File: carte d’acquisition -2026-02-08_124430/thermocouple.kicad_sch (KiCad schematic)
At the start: 6 parts, among them U6 MAX31855SASA_T, U7 MC74HC4067ADWR2G, U8 MC74HC4067ADWR2G

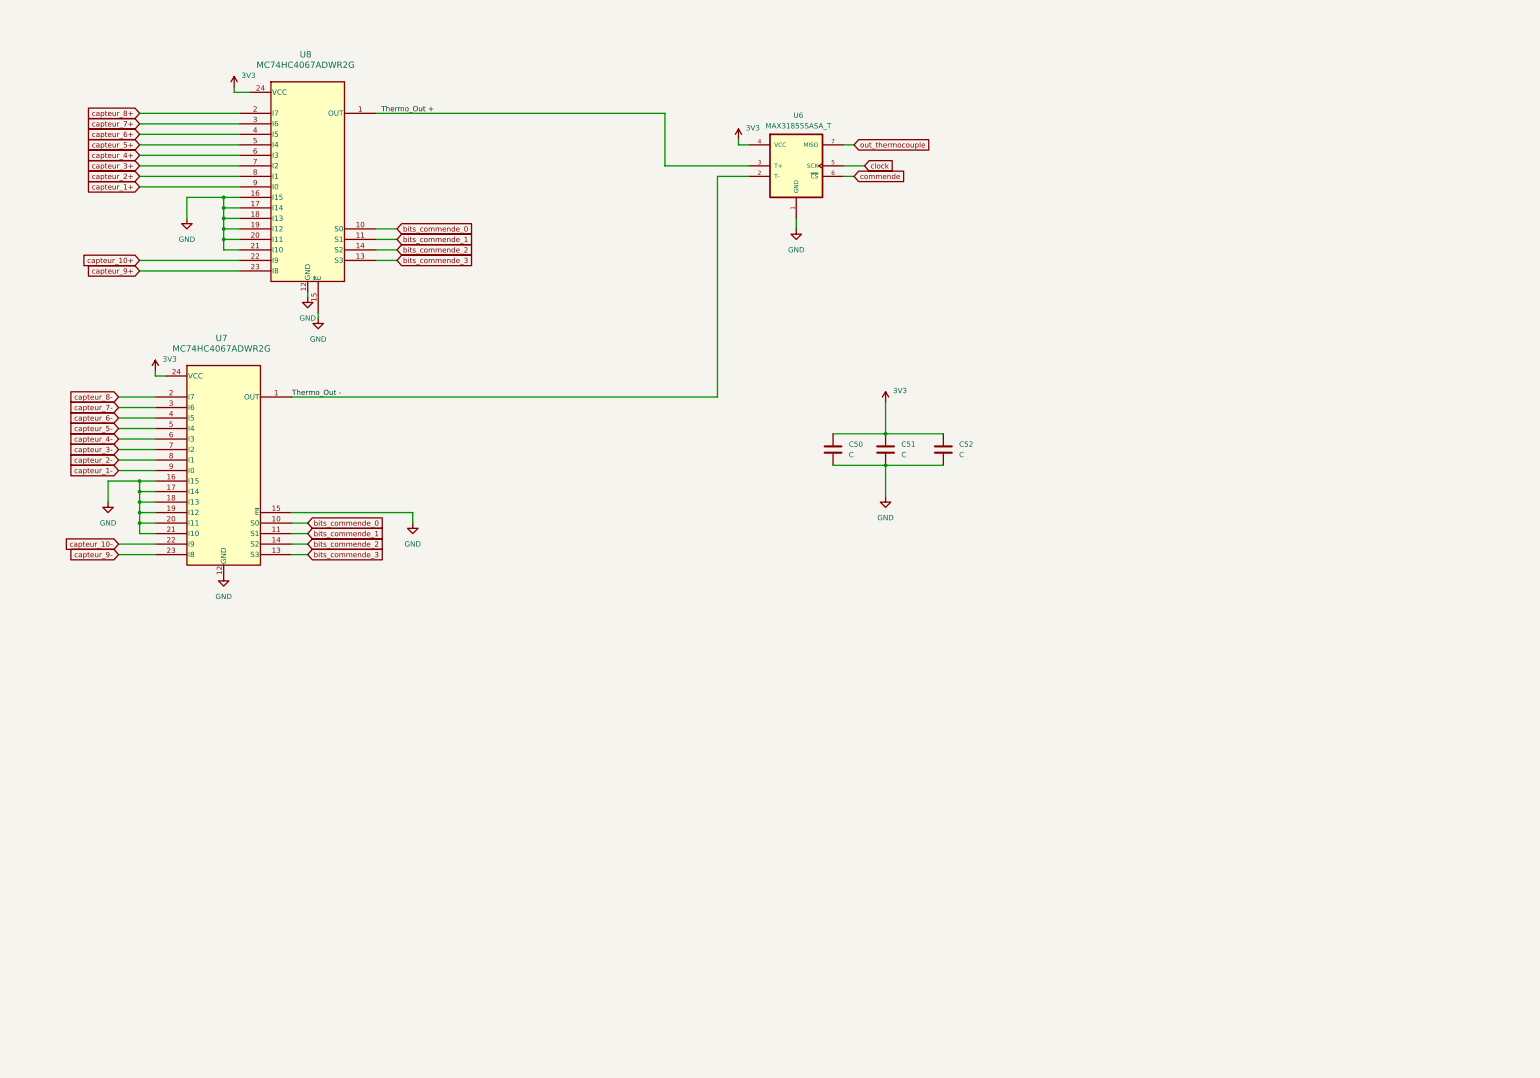
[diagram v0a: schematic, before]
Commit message: arthur net
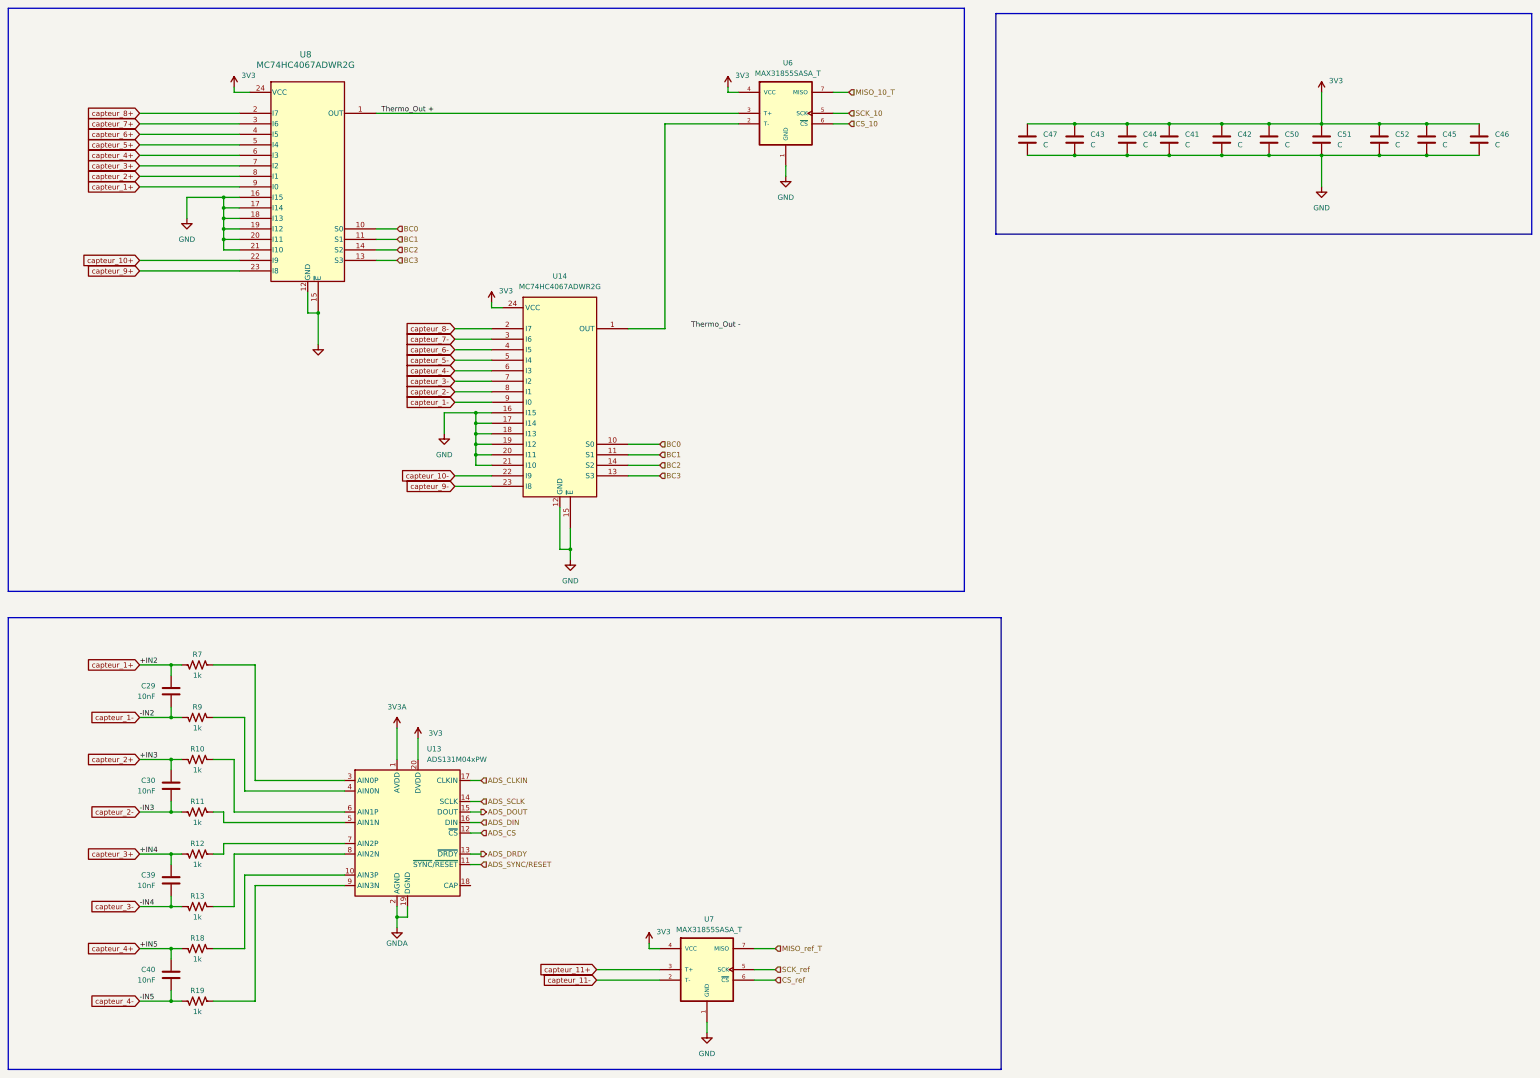
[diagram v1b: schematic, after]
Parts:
- removed U7: MC74HC4067ADWR2G, footprints:SOIC-24WB_ONS, symbol MC74HC4067ADWR2G:MC74HC4067ADWR2G
- added C29, C30, C39, C40: 10nF, symbol Device:C
- added C41, C42, C43, C44, C45, C46, C47: C, symbol Device:C
- added R10, R11, R12, R13, R18, R19, R7, R9: 1k, symbol Device:R_US
- added U13: ADS131M04xPW, Package_SO:TSSOP-20_4.4x6.5mm_P0.65mm, symbol Analog_ADC:ADS131M04xPW
- added U14: MC74HC4067ADWR2G, Package_SO:SOIC-24W_7.5x15.4mm_P1.27mm, symbol FSU_LIB:MC74HC406
- added U7: MAX31855SASA_T, MAX31855SASA_T:SOIC127P600X175-8N, symbol MAX31855SASA_T:MAX31855SASA_T
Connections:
- net 3V3: now also C41.1, C42.1, C43.1, C44.1, C45.1, C46.1, C47.1, U13.20 (DVDD), U14.24 (VCC), U7.4 (VCC)
- net GND: now also C41.2, C42.2, C43.2, C44.2, C45.2, C46.2, C47.2, U14.12 (GND), U14.15 (~{E}), U14.16 (I15), U14.17 (I14), U14.18 (I13), U14.19 (I12), U14.20 (I11), U14.21 (I10), U7.1 (GND)
- net Thermo_Out -: no longer U6.2 (T-)
- net capteur_1+: now also C29.2, R7.2
- net capteur_1-: now also C29.1, R9.2, U14.9 (I0)
- net capteur_10-: now also U14.22 (I9)
- net capteur_2+: now also C30.2, R10.2
- net capteur_2-: now also C30.1, R11.2, U14.8 (I1)
- net capteur_3+: now also C39.2, R12.2
- net capteur_3-: now also C39.1, R13.2, U14.7 (I2)
- net capteur_4+: now also C40.2, R18.2
- net capteur_4-: now also C40.1, R19.2, U14.6 (I3)
- net capteur_5-: now also U14.5 (I4)
- net capteur_6-: now also U14.4 (I5)
- net capteur_7-: now also U14.3 (I6)
- net capteur_8-: now also U14.2 (I7)
- net capteur_9-: now also U14.23 (I8)
- net bits_commende_0 renamed BC0
- net BC0: now also U14.10 (S0)
- net bits_commende_1 renamed BC1
- net BC1: now also U14.11 (S1)
- net bits_commende_2 renamed BC2
- net BC2: now also U14.14 (S2)
- net bits_commende_3 renamed BC3
- net BC3: now also U14.13 (S3)
- net clock renamed SCK_10
- net commende renamed CS_10
- net out_thermocouple renamed MISO_10_T
- new net: R7.1, U13.3 (AIN0P)
- new net: R18.1, U13.10 (AIN3P)
- new net: R9.1, U13.4 (AIN0N)
- new net: R11.1, U13.5 (AIN1N)
- new net: R10.1, U13.6 (AIN1P)
- new net: R12.1, U13.7 (AIN2P)
- new net: R13.1, U13.8 (AIN2N)
- new net: R19.1, U13.9 (AIN3N)
- new net: U14.1 (OUT), U6.2 (T-)
- new net 3V3A: U13.1 (AVDD)
- new net ADS_CLKIN: U13.17 (CLKIN)
- new net ADS_CS: U13.12 (~{CS})
- new net ADS_DIN: U13.16 (DIN)
- new net ADS_DOUT: U13.15 (DOUT)
- new net ADS_DRDY: U13.13 (~{DRDY})
- new net ADS_SCLK: U13.14 (SCLK)
- new net ADS_SYNC/RESET: U13.11 (~{SYNC}/~{RESET})
- new net CS_ref: U7.6 (~{CS})
- new net GNDA: U13.19 (DGND), U13.2 (AGND)
- new net MISO_ref_T: U7.7 (MISO)
- new net SCK_ref: U7.5 (SCK)
- new net capteur_11+: U7.3 (T+)
- new net capteur_11-: U7.2 (T-)
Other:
- moved on the sheet: C50, C51, C52, U6
